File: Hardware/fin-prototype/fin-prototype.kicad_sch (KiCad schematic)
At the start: 88 parts, among them J1 USB_C_Receptacle_USB2.0_16P, J10 Conn_01x01_Pin, J11 Conn_01x01_Pin, J12 Conn_01x01_Pin, J13 Conn_01x01_Pin, J14 Conn_01x01_Pin, J15 Conn_01x01_Pin, J16 Conn_01x01_Pin, J17 Conn_01x01_Pin, J18 Conn_01x01_Pin, J2 Conn_01x04_Pin, J3 Conn_01x04_Pin, J4 Conn_01x08_Pin, J5 Conn_01x04_Pin, J6 Conn_01x01_Pin, J7 Conn_01x01_Pin, J8 Conn_01x01_Pin, J9 Conn_01x01_Pin, SW1 SW_Push, SW2 SW_Push, U1 ADS131M03QPWRQ1, U2 STM32L412C8Tx, U3 W25N512GVEIG, U4 TMP235A4DBZR, U5 FT232RNQ-REEL

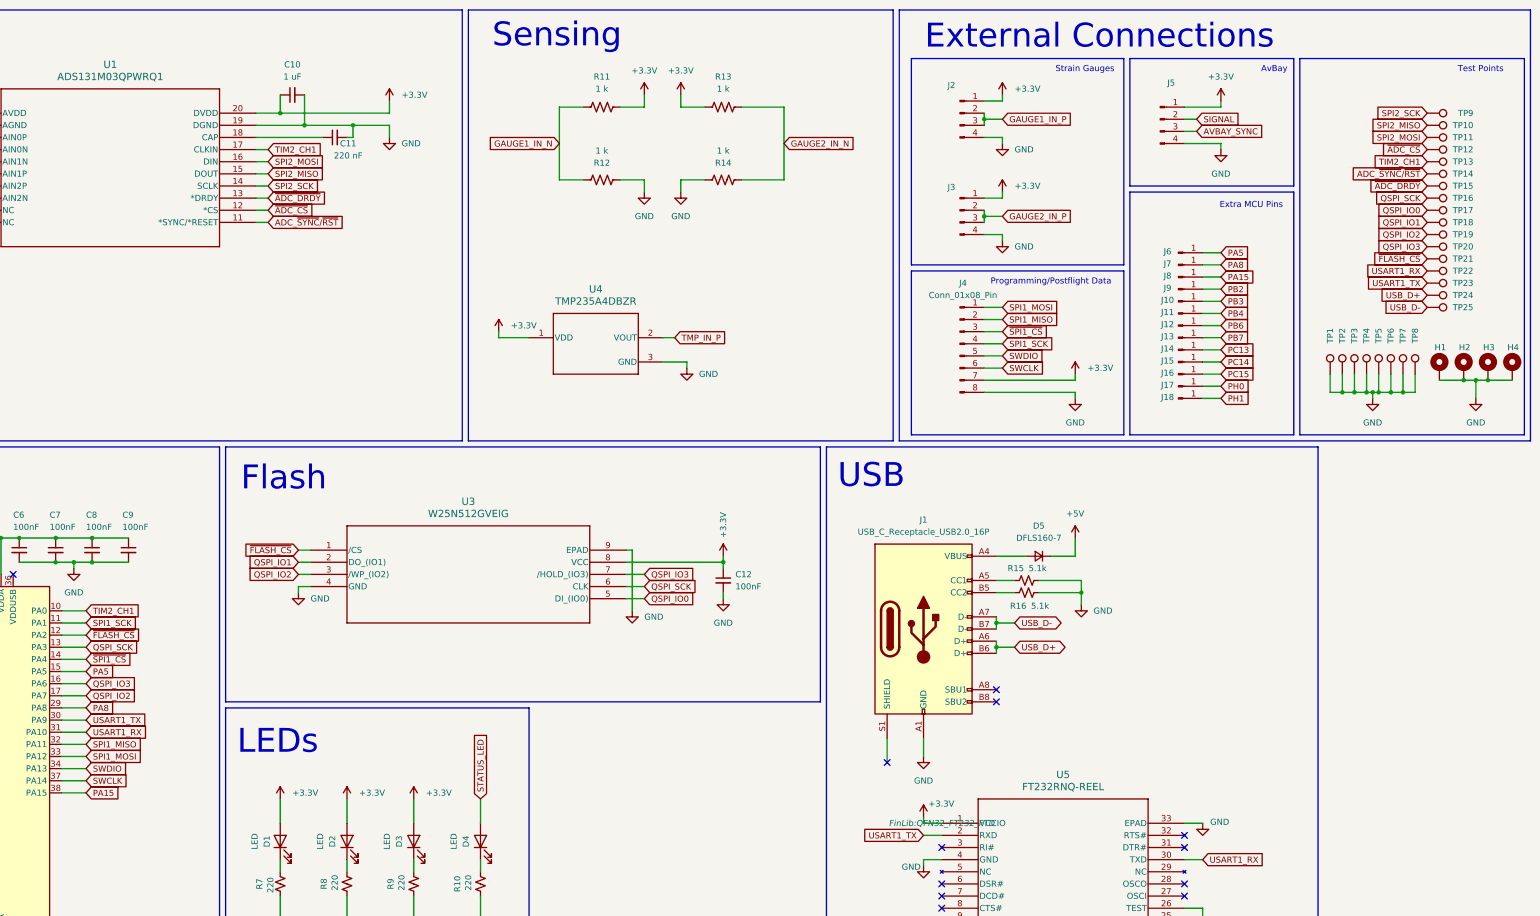
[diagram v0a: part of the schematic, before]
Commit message: Revert "place more components and silkscreen"
This reverts commit 1bc8328d4b62153ca3fb5bb472924e08519ee507.
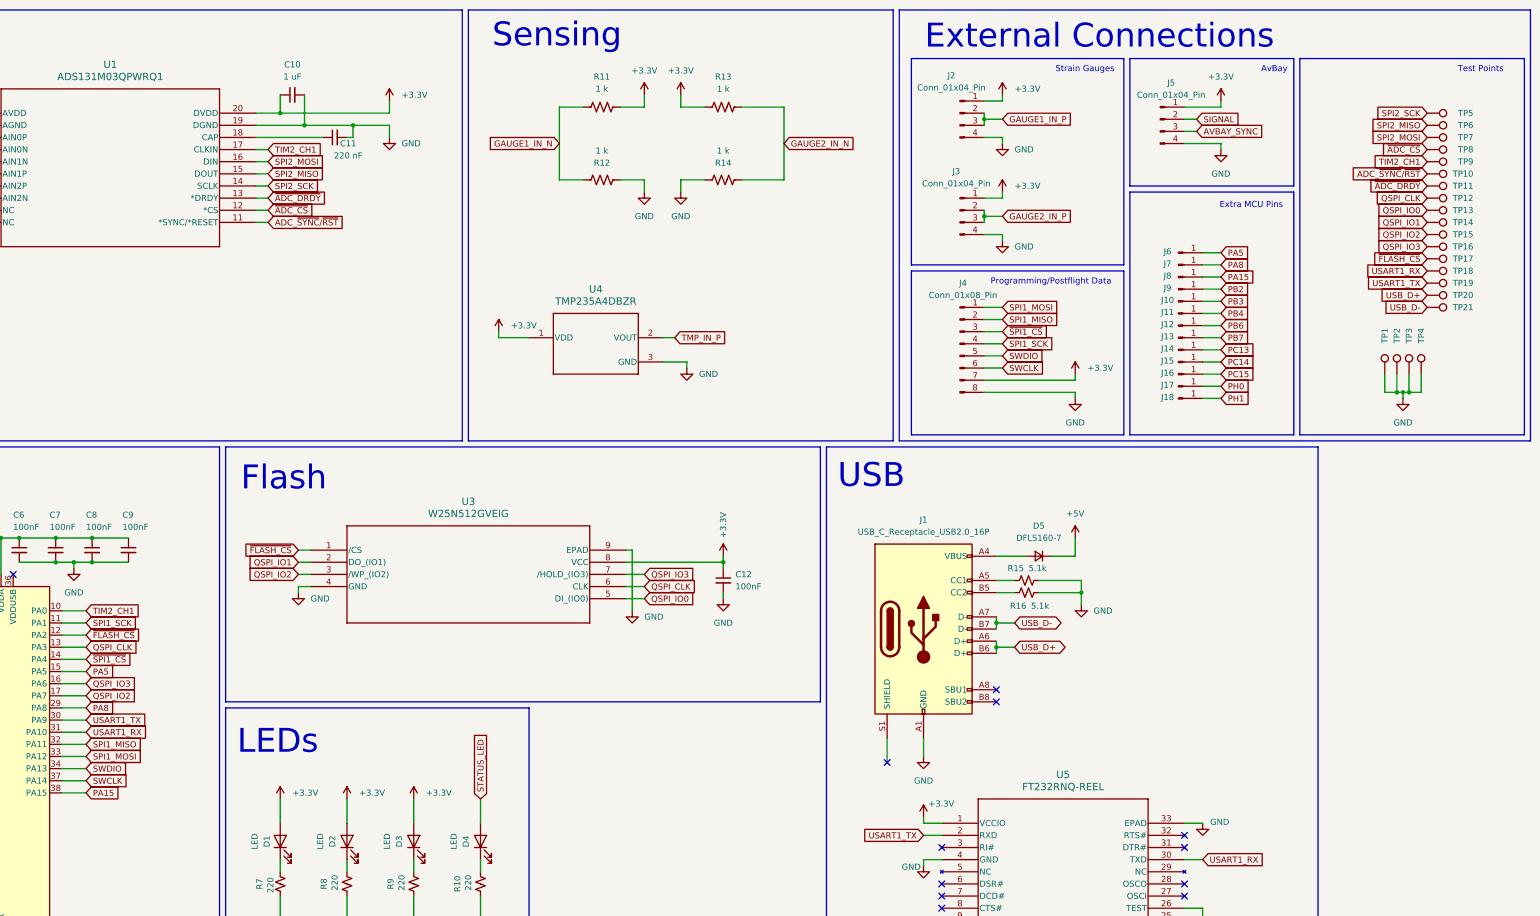
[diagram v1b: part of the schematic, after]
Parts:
- removed H1, H2, H3, H4: MountingHole_Pad, MountingHole:MountingHole_2.2mm_M2_Pad, symbol Mechanical:MountingHole_Pad
- removed TP5, TP6, TP7, TP8: TestPoint, Connector_PinSocket_2.54mm:PinSocket_1x01_P2.54mm_Vertical, symbol Connector:TestPoint
- D1: Signal PWR -> (none)
- D2: Signal TX -> (none)
- D3: Signal RX -> (none)
- D4: Signal STATUS -> (none)
- J10: footprint FinLib:SimpleThroughHole -> Connector_PinHeader_2.54mm:PinHeader_1x01_P2.54mm_Vertical; MCU Pin PB3 -> (none)
- J11: footprint FinLib:SimpleThroughHole -> Connector_PinHeader_2.54mm:PinHeader_1x01_P2.54mm_Vertical; MCU Pin PB4 -> (none)
- J12: footprint FinLib:SimpleThroughHole -> Connector_PinHeader_2.54mm:PinHeader_1x01_P2.54mm_Vertical; MCU Pin PB6 -> (none)
- J13: footprint FinLib:SimpleThroughHole -> Connector_PinHeader_2.54mm:PinHeader_1x01_P2.54mm_Vertical; MCU Pin PB7 -> (none)
- J14: footprint FinLib:SimpleThroughHole -> Connector_PinHeader_2.54mm:PinHeader_1x01_P2.54mm_Vertical; MCU Pin PC13 -> (none)
- J15: footprint FinLib:SimpleThroughHole -> Connector_PinHeader_2.54mm:PinHeader_1x01_P2.54mm_Vertical; MCU Pin PC14 -> (none)
- J16: footprint FinLib:SimpleThroughHole -> Connector_PinHeader_2.54mm:PinHeader_1x01_P2.54mm_Vertical; MCU Pin PC15 -> (none)
- J17: footprint FinLib:SimpleThroughHole -> Connector_PinHeader_2.54mm:PinHeader_1x01_P2.54mm_Vertical; MCU Pin PH0 -> (none)
- J18: footprint FinLib:SimpleThroughHole -> Connector_PinHeader_2.54mm:PinHeader_1x01_P2.54mm_Vertical; MCU Pin PH1 -> (none)
- J2: ADC Channel CH2 -> (none)
- J3: ADC Channel CH1 -> (none)
- J6: footprint FinLib:SimpleThroughHole -> Connector_PinHeader_2.54mm:PinHeader_1x01_P2.54mm_Vertical; MCU Pin PA5 -> (none)
- J7: footprint FinLib:SimpleThroughHole -> Connector_PinHeader_2.54mm:PinHeader_1x01_P2.54mm_Vertical; MCU Pin PA8 -> (none)
- J8: footprint FinLib:SimpleThroughHole -> Connector_PinHeader_2.54mm:PinHeader_1x01_P2.54mm_Vertical; MCU Pin PA15 -> (none)
- J9: footprint FinLib:SimpleThroughHole -> Connector_PinHeader_2.54mm:PinHeader_1x01_P2.54mm_Vertical; MCU Pin PB2 -> (none)
- TP1, TP2, TP3, TP4: footprint Connector_PinHeader_2.54mm:PinHeader_1x01_P2.54mm_Vertical -> TestPoint:TestPoint_Loop_D1.80mm_Drill1.0mm_Beaded
- TP10: renamed from TP14; Signal RST -> (none)
- TP11: renamed from TP15; Signal DRDY -> (none)
- TP12: renamed from TP16; Signal SCK -> (none)
- TP13: renamed from TP17; Signal IO0 -> (none)
- TP14: renamed from TP18; Signal IO1 -> (none)
- TP15: renamed from TP19; Signal IO2 -> (none)
- TP16: renamed from TP20; Signal IO3 -> (none)
- TP18: renamed from TP22; Signal RX -> (none)
- TP19: renamed from TP23; Signal TX -> (none)
- TP20: renamed from TP24; Signal USB+ -> (none)
- TP21: renamed from TP25; Signal USB- -> (none)
- TP5: renamed from TP9; Signal SCK -> (none)
- TP6: renamed from TP10; Signal MISO -> (none)
- TP7: renamed from TP11; Signal MOSI -> (none)
- TP8: renamed from TP12; Signal CS -> (none)
- TP9: renamed from TP13; Signal CLK -> (none)
- renumbered TP21 to TP17
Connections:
- net QSPI_SCK renamed QSPI_CLK
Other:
- moved on the sheet: TP1, TP2, TP3, TP4
